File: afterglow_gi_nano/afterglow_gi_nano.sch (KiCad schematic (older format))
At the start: 53 parts, among them J1 Conn_02x17_Odd_Even, J2 POWER_CONN, J3 GI_WPC_J120, J4 GI_WPC_J121, J5 GI_CONN_J119, J6 Conn_02x17_Odd_Even, Q1 FQP30N06L, Q2 FQP30N06L, Q3 FQP30N06L, Q4 FQP30N06L, Q5 FQP30N06L, U1 74LS374, U2 L7805

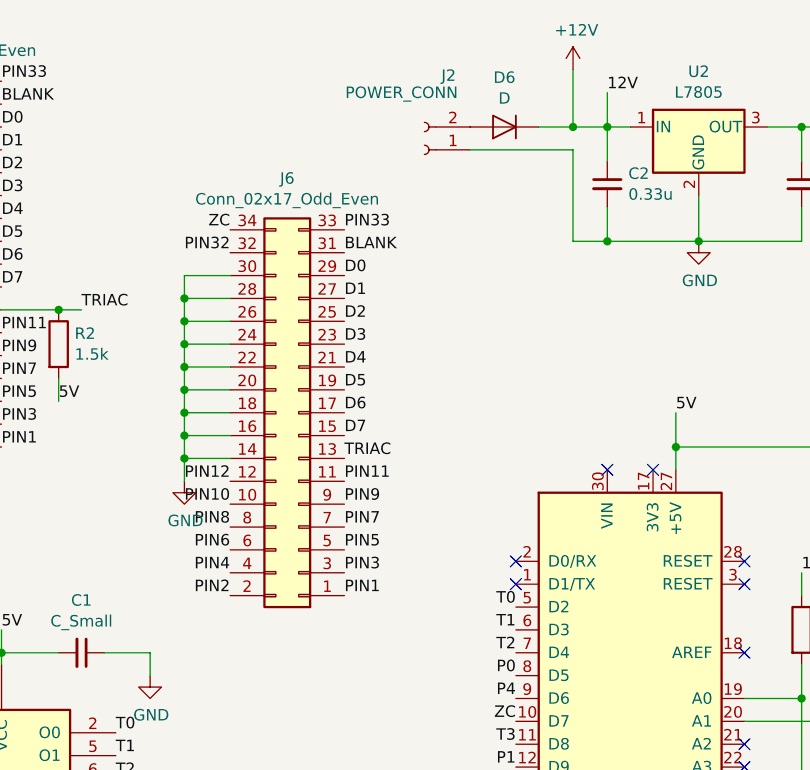
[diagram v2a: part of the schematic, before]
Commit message: Designing the PCB
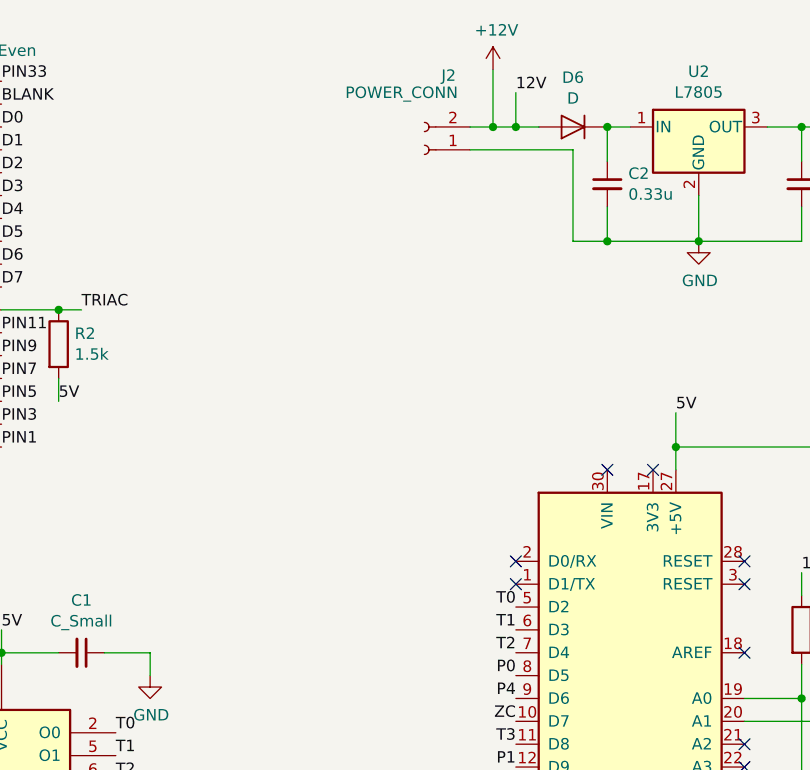
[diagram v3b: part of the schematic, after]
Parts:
- removed J6: Conn_02x17_Odd_Even, Pin_Headers:Pin_Header_Straight_2x17_Pitch2.54mm, symbol Connector_Generic:Conn_02x17_Odd_Even
- J2: footprint Connectors_Molex:Molex_KK-41791-02_02x3.96mm_Straight -> Connectors_Terminal_Blocks:TerminalBlock_Philmore_TB132_02x5mm_Straight
- U1: footprint Housings_DIP:DIP-20_W7.62mm_LongPads -> Housings_SOIC:SOIC-20W_7.5x12.8mm_Pitch1.27mm
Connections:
- net +12V: now also D6.2 (A), J2.2 (Pin_2); no longer C2.1, D6.1 (K), U2.1 (IN)
- new net: C2.1, D6.1 (K), U2.1 (IN)
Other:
- moved on the sheet: D6
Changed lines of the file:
@@
 F 0 "U1" H 1400 5350 50  0000 C CNN
 F 1 "74LS374" H 1400 5250 50  0000 C CNN
-F 2 "Housings_DIP:DIP-20_W7.62mm_LongPads" H 1750 4400 50  0001 C CNN
+F 2 "Housings_SOIC:SOIC-20W_7.5x12.8mm_Pitch1.27mm" H 1750 4400 50  0001 C CNN
 F 3 "http://www.ti.com/lit/gpn/sn74LS374" H 1750 4400 50  0001 C CNN
 	1    1750 4400
@@
 F 0 "J2" H 3494 1025 50  0000 C CNN
 F 1 "POWER_CONN" H 3700 1100 50  0000 C CNN
-F 2 "Connectors_Molex:Molex_KK-41791-02_02x3.96mm_Straight" H 3600 1350 50  0001 C CNN
+F 2 "Connectors_Terminal_Blocks:TerminalBlock_Philmore_TB132_02x5mm_Straight" H 3600 1350 50  0001 C CNN
 F 3 "~" H 3600 1350 50  0001 C CNN
 	1    3600 1350
@@
 L power:+12V #PWR0104
 U 1 1 5C2FAA66
-P 4250 1000
-F 0 "#PWR0104" H 4250 850 50  0001 C CNN
-F 1 "+12V" H 4265 1173 50  0000 C CNN
-F 2 "" H 4250 1000 50  0001 C CNN
-F 3 "" H 4250 1000 50  0001 C CNN
-	1    4250 1000
+P 3900 1000
+F 0 "#PWR0104" H 3900 850 50  0001 C CNN
+F 1 "+12V" H 3915 1173 50  0000 C CNN
+F 2 "" H 3900 1000 50  0001 C CNN
+F 3 "" H 3900 1000 50  0001 C CNN
+	1    3900 1000
 	1    0    0    -1
 $EndComp
 Wire Wire Line
-	4100 1250 4250 1250
-Connection ~ 4250 1250
-Wire Wire Line
-	4250 1250 4400 1250
-Wire Wire Line
-	4250 1250 4250 1000
+	3900 1250 3900 1000
 Wire Wire Line
 	4250 1350 4250 1750
@@
 Wire Wire Line
 	4400 1400 4400 1250
-Connection ~ 4400 1250
 Wire Wire Line
 	4400 1250 4500 1250
@@
 T4
 Wire Wire Line
-	4400 1250 4400 1100
-Text Label 4400 1100 0    50   ~ 0
+	4000 1250 4000 1100
+Text Label 4000 1100 0    50   ~ 0
 12V
 $Comp
@@
 L Device:D D6
 U 1 1 5C3DDC36
-P 3950 1250
-F 0 "D6" H 3950 1034 50  0000 C CNN
-F 1 "D" H 3950 1125 50  0000 C CNN
-F 2 "Diodes_THT:D_5W_P10.16mm_Horizontal" H 3950 1250 50  0001 C CNN
-F 3 "~" H 3950 1250 50  0001 C CNN
-	1    3950 1250
+P 4250 1250
+F 0 "D6" H 4250 1034 50  0000 C CNN
+F 1 "D" H 4250 1125 50  0000 C CNN
+F 2 "Diodes_THT:D_5W_P10.16mm_Horizontal" H 4250 1250 50  0001 C CNN
+F 3 "~" H 4250 1250 50  0001 C CNN
+	1    4250 1250
 	-1   0    0    1
 $EndComp
@@
 	1    0    0    -1
 $EndComp
-$Comp
-L Connector_Generic:Conn_02x17_Odd_Even J6
-U 1 1 5C44FDE0
-P 3050 2500
-F 0 "J6" H 3100 1475 50  0000 C CNN
-F 1 "Conn_02x17_Odd_Even" H 3100 1566 50  0000 C CNN
-F 2 "Pin_Headers:Pin_Header_Straight_2x17_Pitch2.54mm" H 3050 2500 50  0001 C CNN
-F 3 "~" H 3050 2500 50  0001 C CNN
-	1    3050 2500
-	-1   0    0    1
-$EndComp
-Text Label 3250 1800 0    50   ~ 0
-BLANK
-Text Label 3250 1900 0    50   ~ 0
-D0
-Text Label 3250 2000 0    50   ~ 0
-D1
-Text Label 3250 2100 0    50   ~ 0
-D2
-Text Label 3250 2200 0    50   ~ 0
-D3
-Text Label 3250 2300 0    50   ~ 0
-D4
-Text Label 3250 2400 0    50   ~ 0
-D5
-Text Label 3250 2500 0    50   ~ 0
-D6
-Text Label 3250 2600 0    50   ~ 0
-D7
-Text Label 3250 2700 0    50   ~ 0
-TRIAC
-Text Label 2750 1700 2    50   ~ 0
-ZC
-Wire Wire Line
-	2750 1900 2550 1900
-Wire Wire Line
-	2550 1900 2550 2000
-Wire Wire Line
-	2550 2700 2750 2700
-Connection ~ 2550 2700
-Wire Wire Line
-	2550 2700 2550 2800
-Wire Wire Line
-	2750 2600 2550 2600
-Connection ~ 2550 2600
-Wire Wire Line
-	2550 2600 2550 2700
-Wire Wire Line
-	2550 2500 2750 2500
-Connection ~ 2550 2500
-Wire Wire Line
-	2550 2500 2550 2600
-Wire Wire Line
-	2750 2400 2550 2400
-Connection ~ 2550 2400
-Wire Wire Line
-	2550 2400 2550 2500
-Wire Wire Line
-	2550 2300 2750 2300
-Connection ~ 2550 2300
-Wire Wire Line
-	2550 2300 2550 2400
-Wire Wire Line
-	2750 2200 2550 2200
-Connection ~ 2550 2200
-Wire Wire Line
-	2550 2200 2550 2300
-Wire Wire Line
-	2550 2100 2750 2100
-Connection ~ 2550 2100
-Wire Wire Line
-	2550 2100 2550 2200
-Wire Wire Line
-	2750 2000 2550 2000
-Connection ~ 2550 2000
-Wire Wire Line
-	2550 2000 2550 2100
-$Comp
-L power:GND #PWR01
-U 1 1 5C44FE0B
-P 2550 2800
-F 0 "#PWR01" H 2550 2550 50  0001 C CNN
-F 1 "GND" H 2555 2627 50  0000 C CNN
-F 2 "" H 2550 2800 50  0001 C CNN
-F 3 "" H 2550 2800 50  0001 C CNN
-	1    2550 2800
-	1    0    0    -1
-$EndComp
 Text Label 1250 1150 2    50   ~ 0
 PIN32
@@
 Text Label 1750 1050 0    50   ~ 0
 PIN33
-Text Label 3250 1700 0    50   ~ 0
-PIN33
-Text Label 3250 2800 0    50   ~ 0
-PIN11
-Text Label 3250 2900 0    50   ~ 0
-PIN9
-Text Label 3250 3000 0    50   ~ 0
-PIN7
-Text Label 3250 3100 0    50   ~ 0
-PIN5
-Text Label 3250 3200 0    50   ~ 0
-PIN3
-Text Label 3250 3300 0    50   ~ 0
-PIN1
-Text Label 2750 2800 2    50   ~ 0
-PIN12
-Text Label 2750 1800 2    50   ~ 0
-PIN32
-Text Label 2750 3000 2    50   ~ 0
-PIN8
-Text Label 2750 2900 2    50   ~ 0
-PIN10
-Text Label 2750 3100 2    50   ~ 0
-PIN6
-Text Label 2750 3200 2    50   ~ 0
-PIN4
-Text Label 2750 3300 2    50   ~ 0
-PIN2
+Wire Wire Line
+	3800 1250 3900 1250
+Connection ~ 3900 1250
+Wire Wire Line
+	3900 1250 4000 1250
+Connection ~ 4000 1250
+Connection ~ 4400 1250
+Wire Wire Line
+	4000 1250 4100 1250
 $EndSCHEMATC

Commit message: Some PCB progress
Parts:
- RV1: footprint Potentiometers:Potentiometer_Trimmer_Piher_PT-6v_Horizontal -> Potentiometers:Potentiometer_Trimmer_Piher_PT-10v10_Horizontal_Px10.0mm_Py5.0mm
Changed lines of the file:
@@
 F 0 "RV1" H 5481 3896 50  0000 R CNN
 F 1 "R_POT_TRIM" H 5481 3805 50  0000 R CNN
-F 2 "Potentiometers:Potentiometer_Trimmer_Piher_PT-6v_Horizontal" H 5550 3850 50  0001 C CNN
+F 2 "Potentiometers:Potentiometer_Trimmer_Piher_PT-10v10_Horizontal_Px10.0mm_Py5.0mm" H 5550 3850 50  0001 C CNN
 F 3 "~" H 5550 3850 50  0001 C CNN
 	1    5550 3850
